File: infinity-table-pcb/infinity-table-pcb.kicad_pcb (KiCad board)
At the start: 2 copper layers, 40 x 48.9 mm, 10 parts, among them J1 PJ-063AH, J2 Conn_01x05_Male, J3 Conn_01x10_Male

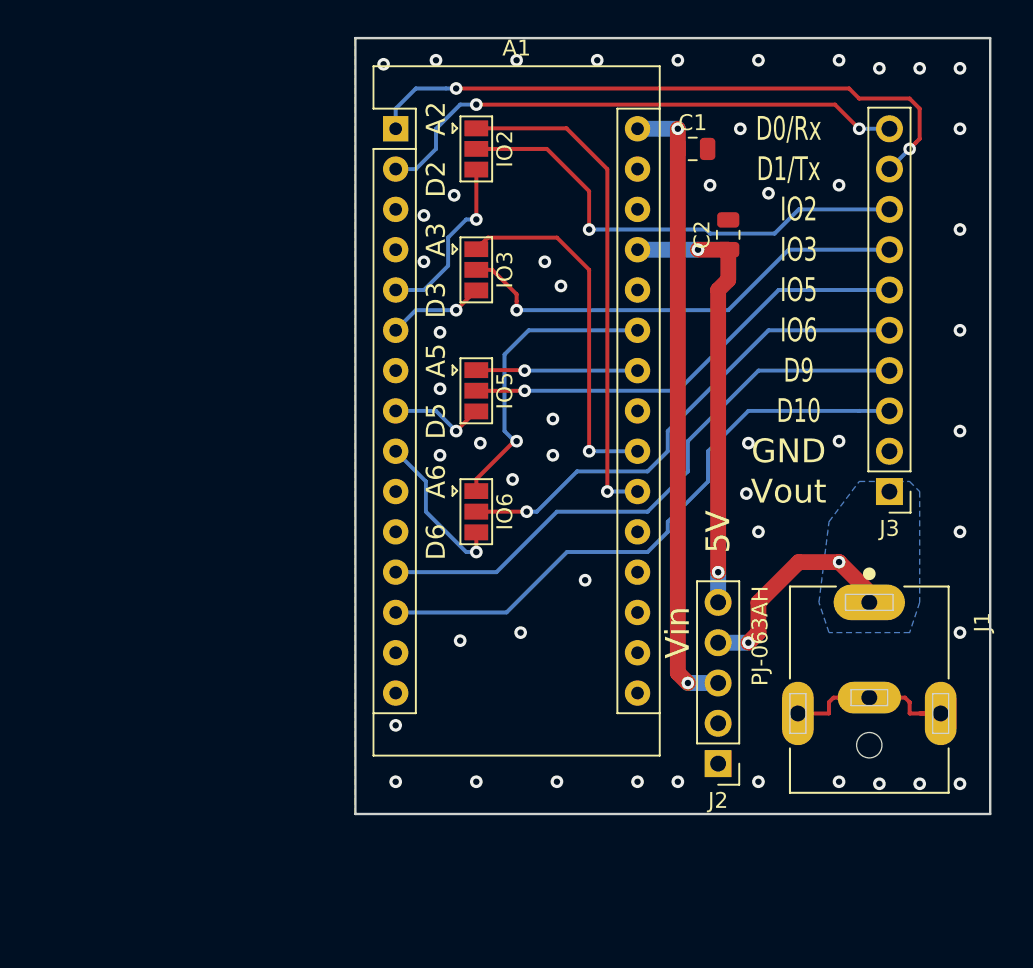
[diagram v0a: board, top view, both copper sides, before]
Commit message: pcb first version done, but need to rework a bit
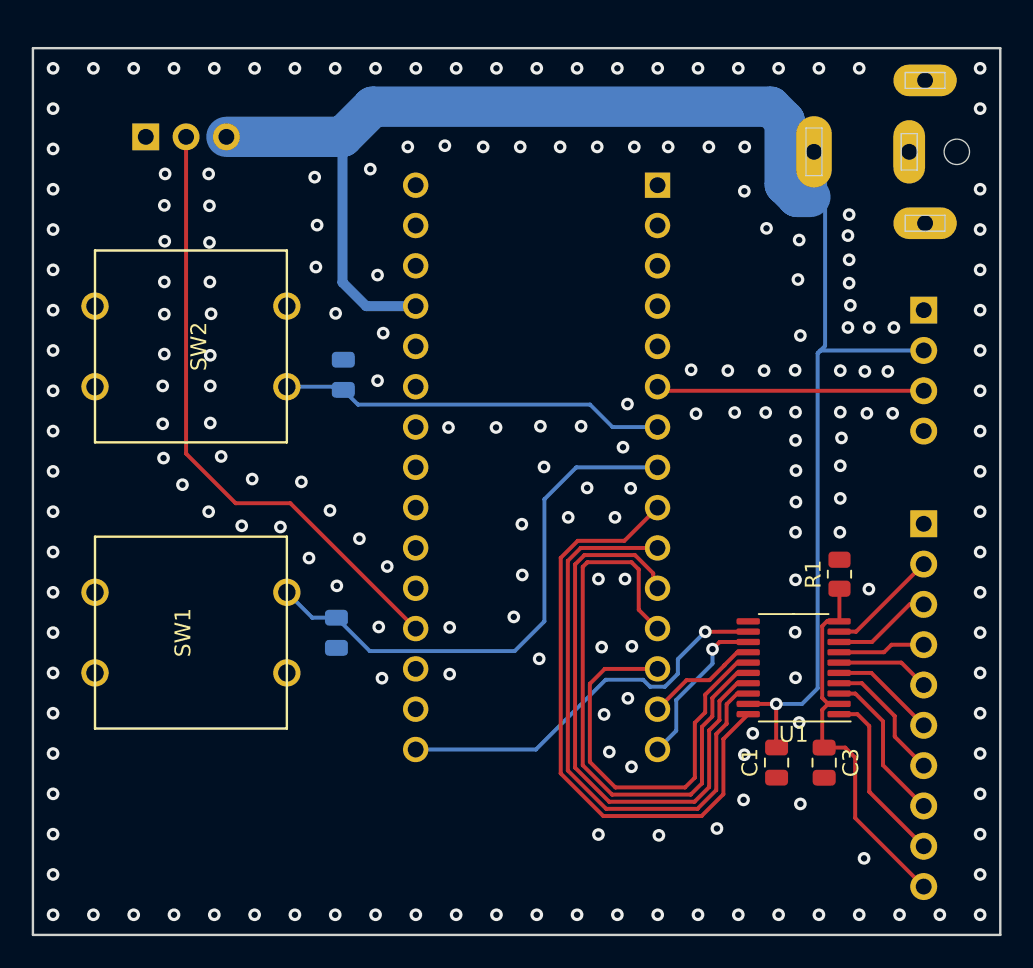
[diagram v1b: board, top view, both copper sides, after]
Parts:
- removed C2: 100nF, Capacitor_SMD:C_0805_2012Metric
- removed IO2, IO3, IO5, IO6: SolderJumper_3_Open, Jumper:SolderJumper-3_P1.3mm_Open_Pad1.0x1.5mm
- added C3: 0,1uF, Capacitor_SMD:C_0805_2012Metric, F.Cu at (156.5, 116.1)
- added C4: 1nF, Capacitor_SMD:C_0805_2012Metric, B.Cu at (125.8, 108.0)
- added C5: 1nF, Capacitor_SMD:C_0805_2012Metric, B.Cu at (126.2, 91.7)
- added R1: R, Resistor_SMD:R_0805_2012Metric, F.Cu at (157.5, 104.3)
- added RV1: R_Potentiometer, Connector_PinHeader_2.54mm:PinHeader_1x03_P2.54mm_Vertical, B.Cu at (113.8, 76.7)
- added SW1: SW_Push_Dual, kicad-ss-libs:Push Button 12x12mm, F.Cu at (116.6, 108.0)
- added SW2: SW_Push_Dual, kicad-ss-libs:Push Button 12x12mm, F.Cu at (116.6, 89.9)
- added U1: TXS0108EPW, Package_SO:TSSOP-20_4.4x6.5mm_P0.65mm, F.Cu at (154.6, 110.2)
- A1, J3: moved to B.Cu
- C1: value 100nF -> 0,1uF
- J1: footprint SS_connectors:CUI_PJ-063AH-1 -> kicad-ss-libs:CUI_PJ-063AH; moved to B.Cu
- J2: value Conn_01x05_Male -> Conn_01x04_Male; footprint Connector_PinHeader_2.54mm:PinHeader_1x05_P2.54mm_Vertical -> Connector_PinHeader_2.54mm:PinHeader_1x04_P2.54mm_Vertical; moved to B.Cu
- moved C1 39.0 mm to (153.5, 116.1), turned to 90 degrees
- moved J2 31.4 mm to (162.8, 87.6)
- moved J1 28.6 mm to (155.9, 77.7), turned to 0 degrees
- moved A1 16.9 mm to (146.0, 79.8), turned to 180 degrees
- moved J3 2.96 mm to (162.8, 101.1)
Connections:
- A1 pad 1: D1 -> unconnected-(A1-Pad1)
- A1 pad 10: (no net) -> Net-(A1-Pad10)
- A1 pad 11: (no net) -> Net-(A1-Pad11)
- A1 pad 12: D9 -> Net-(A1-Pad12)
- A1 pad 13: D10 -> Net-(A1-Pad13)
- A1 pad 14: (no net) -> Net-(A1-Pad14)
- A1 pad 15: (no net) -> Net-(A1-Pad15)
- A1 pad 16: (no net) -> Net-(A1-Pad16)
- A1 pad 17: (no net) -> unconnected-(A1-Pad17)
- A1 pad 18: (no net) -> unconnected-(A1-Pad18)
- A1 pad 19: (no net) -> Net-(A1-Pad19)
- A1 pad 2: D0 -> unconnected-(A1-Pad2)
- A1 pad 20: (no net) -> unconnected-(A1-Pad20)
- A1 pad 21: Net-(A1-Pad21) -> unconnected-(A1-Pad21)
- A1 pad 22: Net-(A1-Pad22) -> unconnected-(A1-Pad22)
- A1 pad 23: (no net) -> unconnected-(A1-Pad23)
- A1 pad 24: Net-(A1-Pad24) -> unconnected-(A1-Pad24)
- A1 pad 25: Net-(A1-Pad25) -> unconnected-(A1-Pad25)
- A1 pad 26: (no net) -> unconnected-(A1-Pad26)
- A1 pad 27: Net-(A1-Pad27) -> +5V
- A1 pad 28: (no net) -> unconnected-(A1-Pad28)
- A1 pad 3: (no net) -> unconnected-(A1-Pad3)
- A1 pad 30: Net-(A1-Pad30) -> unconnected-(A1-Pad30)
- A1 pad 5: D2 -> unconnected-(A1-Pad5)
- A1 pad 6: D3 -> Net-(A1-Pad6)
- A1 pad 7: (no net) -> SW2
- A1 pad 8: D5 -> SW1
- A1 pad 9: D6 -> Net-(A1-Pad9)
- C1 pad 1: Net-(A1-Pad30) -> GND
- C1 pad 2: GND -> +5V
- J1 pad 1: Net-(J1-Pad1) -> +5V
- J2 pad 2: (no net) -> +5V
- J2 pad 3: Net-(A1-Pad30) -> Net-(A1-Pad6)
- J2 pad 4: Net-(J1-Pad1) -> unconnected-(J2-Pad4)
- J3 pad 1: Net-(J1-Pad1) -> GND
- J3 pad 10: D0 -> Net-(C3-Pad1)
- J3 pad 2: GND -> Net-(J3-Pad2)
- J3 pad 3: D10 -> Net-(J3-Pad3)
- J3 pad 4: D9 -> Net-(J3-Pad4)
- J3 pad 9: D1 -> Net-(J3-Pad9)
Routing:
- net +5V: track 0.00 -> 105.2 mm, vias 0 -> 1
- net D1: track 39.9 -> 0.00 mm, vias 2 -> 0
- net Net-(A1-Pad30): track 39.6 -> 0.00 mm, vias 2 -> 0
- net Net-(A1-Pad19): track 0.00 -> 39.0 mm
- net Net-(A1-Pad9): track 0.00 -> 38.6 mm
- net D10: track 37.9 -> 0.00 mm
- net Net-(A1-Pad12): track 0.00 -> 37.7 mm
- net D9: track 37.5 -> 0.00 mm
- net Net-(A1-Pad10): track 0.00 -> 37.4 mm
- net Net-(A1-Pad11): track 0.00 -> 37.2 mm
- net SW1: track 0.00 -> 34.2 mm
- net D0: track 34.2 -> 0.00 mm, vias 2 -> 0
- net Net-(A1-Pad21): track 31.5 -> 0.00 mm, vias 1 -> 0
- net Net-(A1-Pad27): track 28.2 -> 0.00 mm, vias 2 -> 0
- net Net-(A1-Pad13): track 0.00 -> 26.2 mm
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- removed copper zone on B.Cu, net Net-(J1-Pad1)
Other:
- board size 40 x 48.9 mm -> 61 x 55.9 mm
- net class Default removed
- board text removed: "5V"
- board text removed: "A2"
- board text removed: "A3"
- board text removed: "A5"
- board text removed: "A6"
- board text removed: "D0/Rx"
- board text removed: "D1/Tx"
- board text removed: "D10"
- board text removed: "D2"
- board text removed: "D3"
- board text removed: "D5"
- board text removed: "D6"
- board text removed: "D9"
- board text removed: "GND"
- board text removed: "IO2"
- board text removed: "IO3"
- board text removed: "IO5"
- board text removed: "IO6"
- board text removed: "Sami Sorell"
- board text removed: "Tiny Arduino Breakout Board"
- board text removed: "Vin"
- board text removed: "Vout"
